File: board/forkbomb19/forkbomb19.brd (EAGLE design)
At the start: 89.2 x 57 mm, 65 parts, among them SW1 SPST_TACT-KMR2, T3 MMUN2133LT1G, U1 ESP-WROOM-03, U4 TPS61090RSAR, U5 MCP73871, X3 POT_GND, X4 POT_3V3, X5 POT_SIG

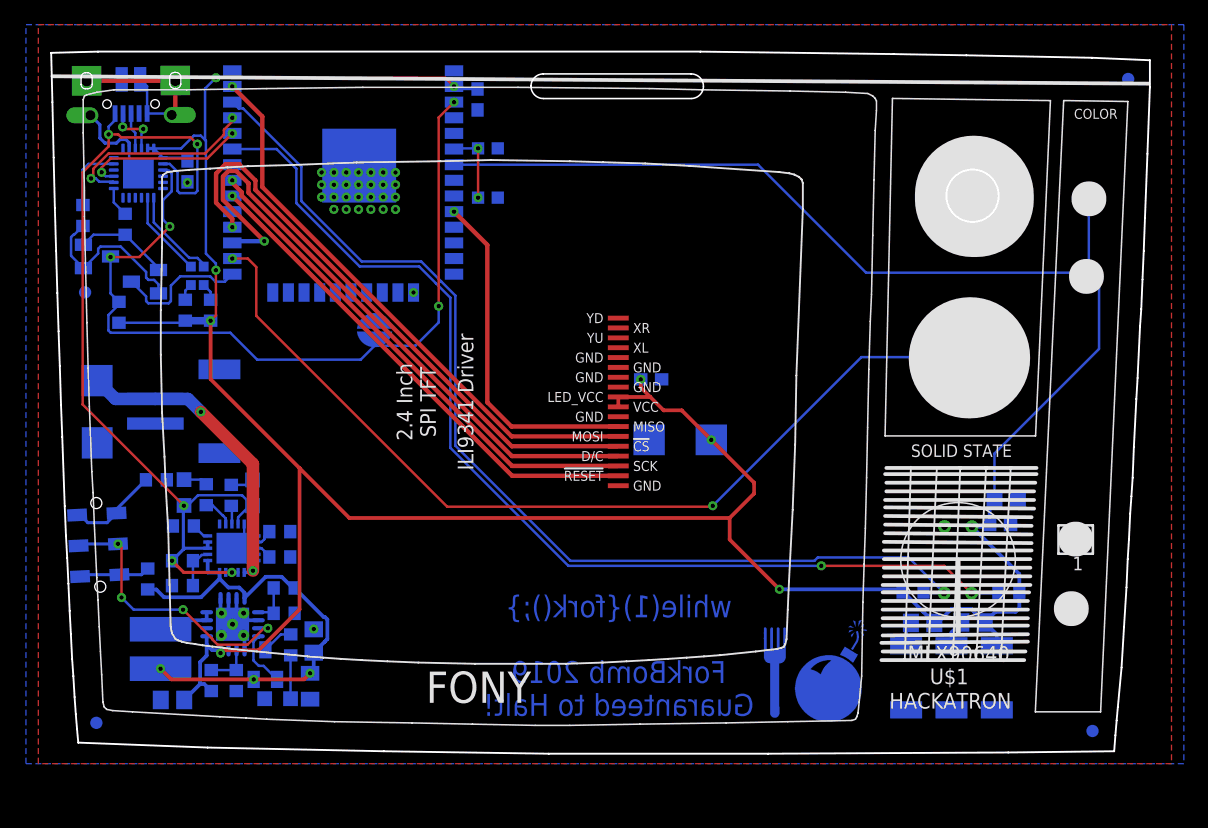
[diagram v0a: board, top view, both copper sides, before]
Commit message: small cleanup
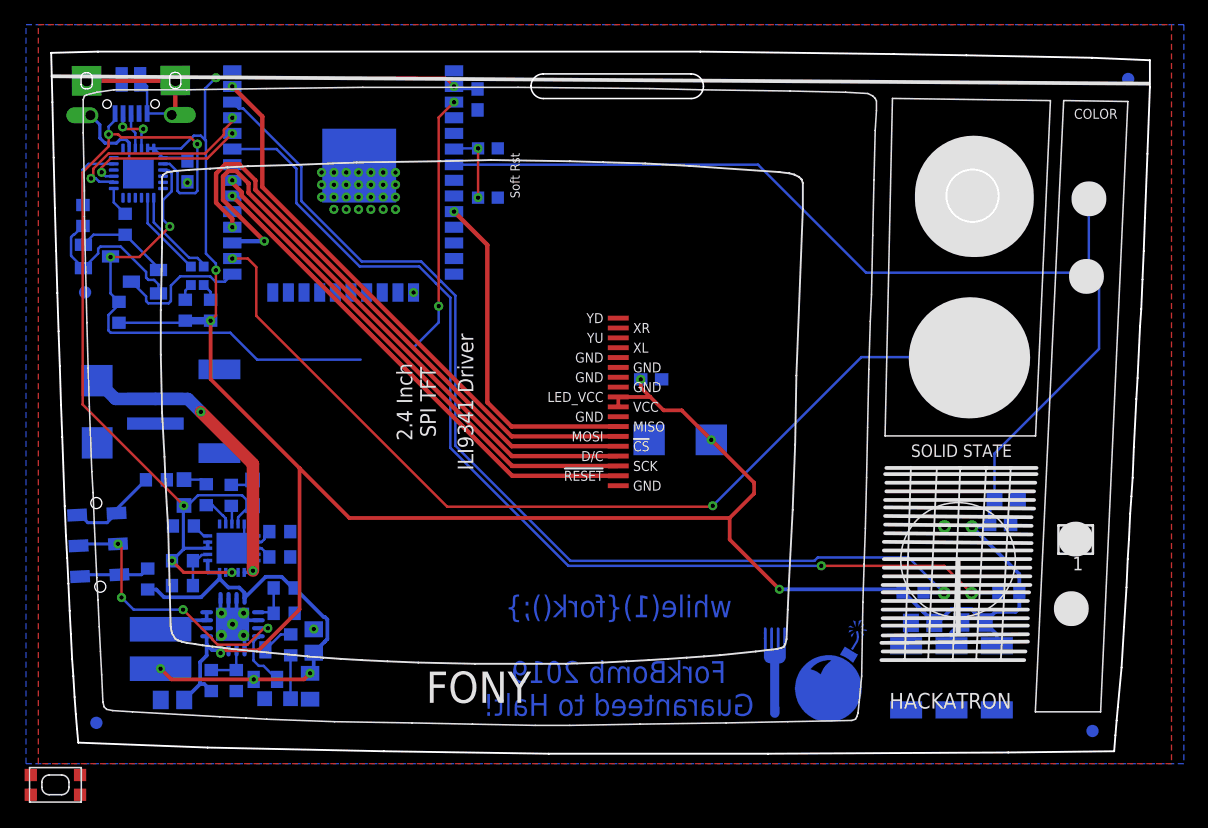
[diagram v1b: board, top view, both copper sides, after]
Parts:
- removed HRDRST: (no value), SparkFun-Jumpers:SMT-JUMPER_2_NO_SILK_ROUND
- added SW2: SPST_TACT-KMR2, adafruit:KMR2
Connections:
- net EN: now also SW2.2, SW2.4; no longer HRDRST.2
- net GND: now also SW2.1, SW2.3; no longer HRDRST.1
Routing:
- net EN: track 65.6 -> 60.7 mm
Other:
- board text added: "Soft Rst"
